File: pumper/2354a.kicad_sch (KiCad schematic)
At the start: 33 parts, among them SW1 1TS015A-1400-0600-CT, SW2 1TS015A-1400-0600-CT, U4 RP2354A-QFN60, U5 ABM8-272-T3_C20625731

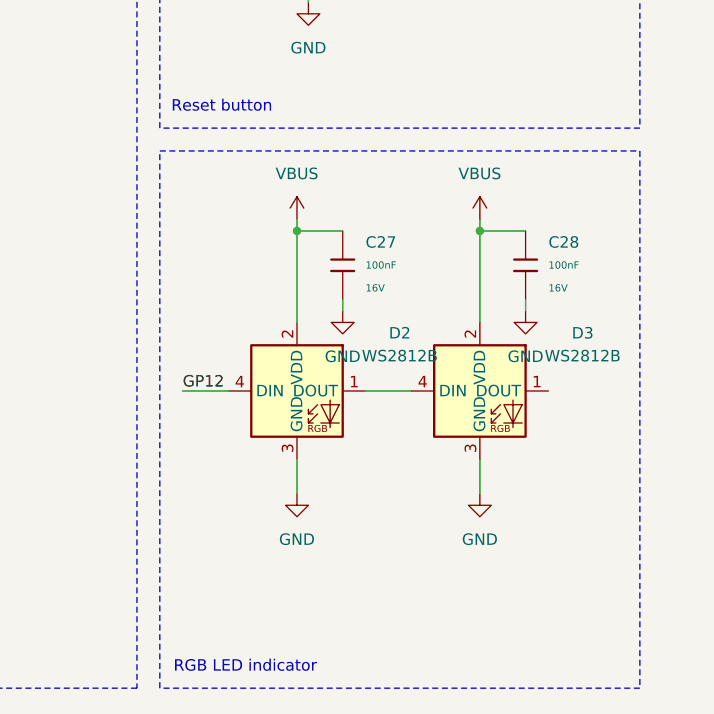
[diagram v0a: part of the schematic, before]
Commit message: feat: update kicad files
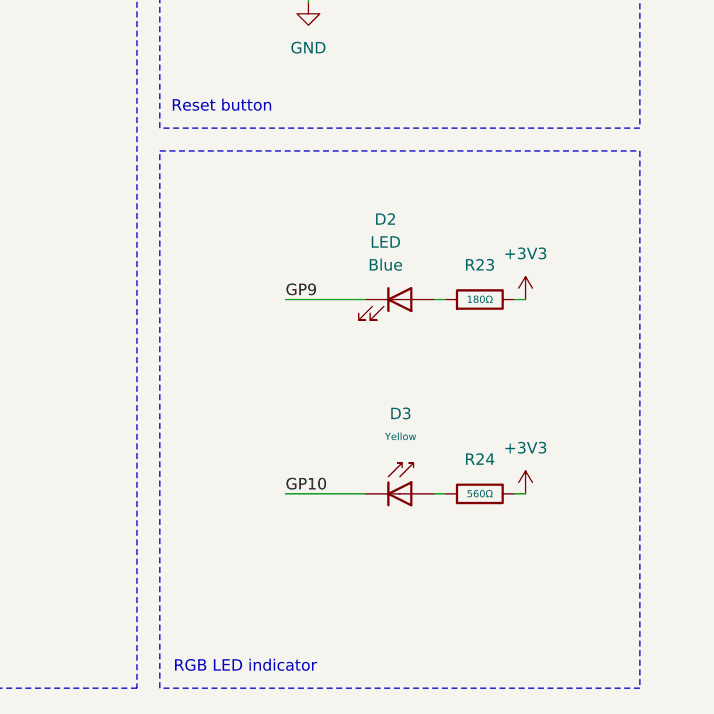
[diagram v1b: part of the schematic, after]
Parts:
- removed C27, C28: 100nF, PCM_JLCPCB:C_0402, symbol PCM_JLCPCB-Capacitors:0402,100nF
- removed D2, D3: WS2812B, PCM_JLCPCB:LED-SMD_4P-L1.6-W1.5_XL-1615RGBC-WS2812B, symbol PCM_JLCPCB-Extended:LED, WS2812B, 1615
- added D2: LED, PCM_JLCPCB:D_0603, symbol Device:LED
- added D3: Yellow, PCM_JLCPCB:D_0603, symbol PCM_JLCPCB-Diodes:LED,0603,Yellow
- added R23: 180Ω, PCM_JLCPCB:R_0603, symbol PCM_JLCPCB-Resistors:0603,180Ω
- added R24: 560Ω, PCM_JLCPCB:R_0603, symbol PCM_JLCPCB-Resistors:0603,560Ω
- TP8, TP9: footprint TestPoint:TestPoint_Pad_D1.5mm -> TestPoint:TestPoint_Pad_D1.0mm
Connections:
- net +3V3: now also R23.2, R24.2
- net GP10: now also D3.1
- net GP9: now also D2.1 (K)
- new net: D3.2, R24.1
- new net: D2.2 (A), R23.1
